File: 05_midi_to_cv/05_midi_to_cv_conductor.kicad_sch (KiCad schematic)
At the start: 21 parts, among them J1 MIDI IN 1, J2 MIDI IN 2, J3 MIDI IN 3, J5 Midi Fast Bus, U1 NCP1117-5.0_SOT223, U2 SN74HCT125

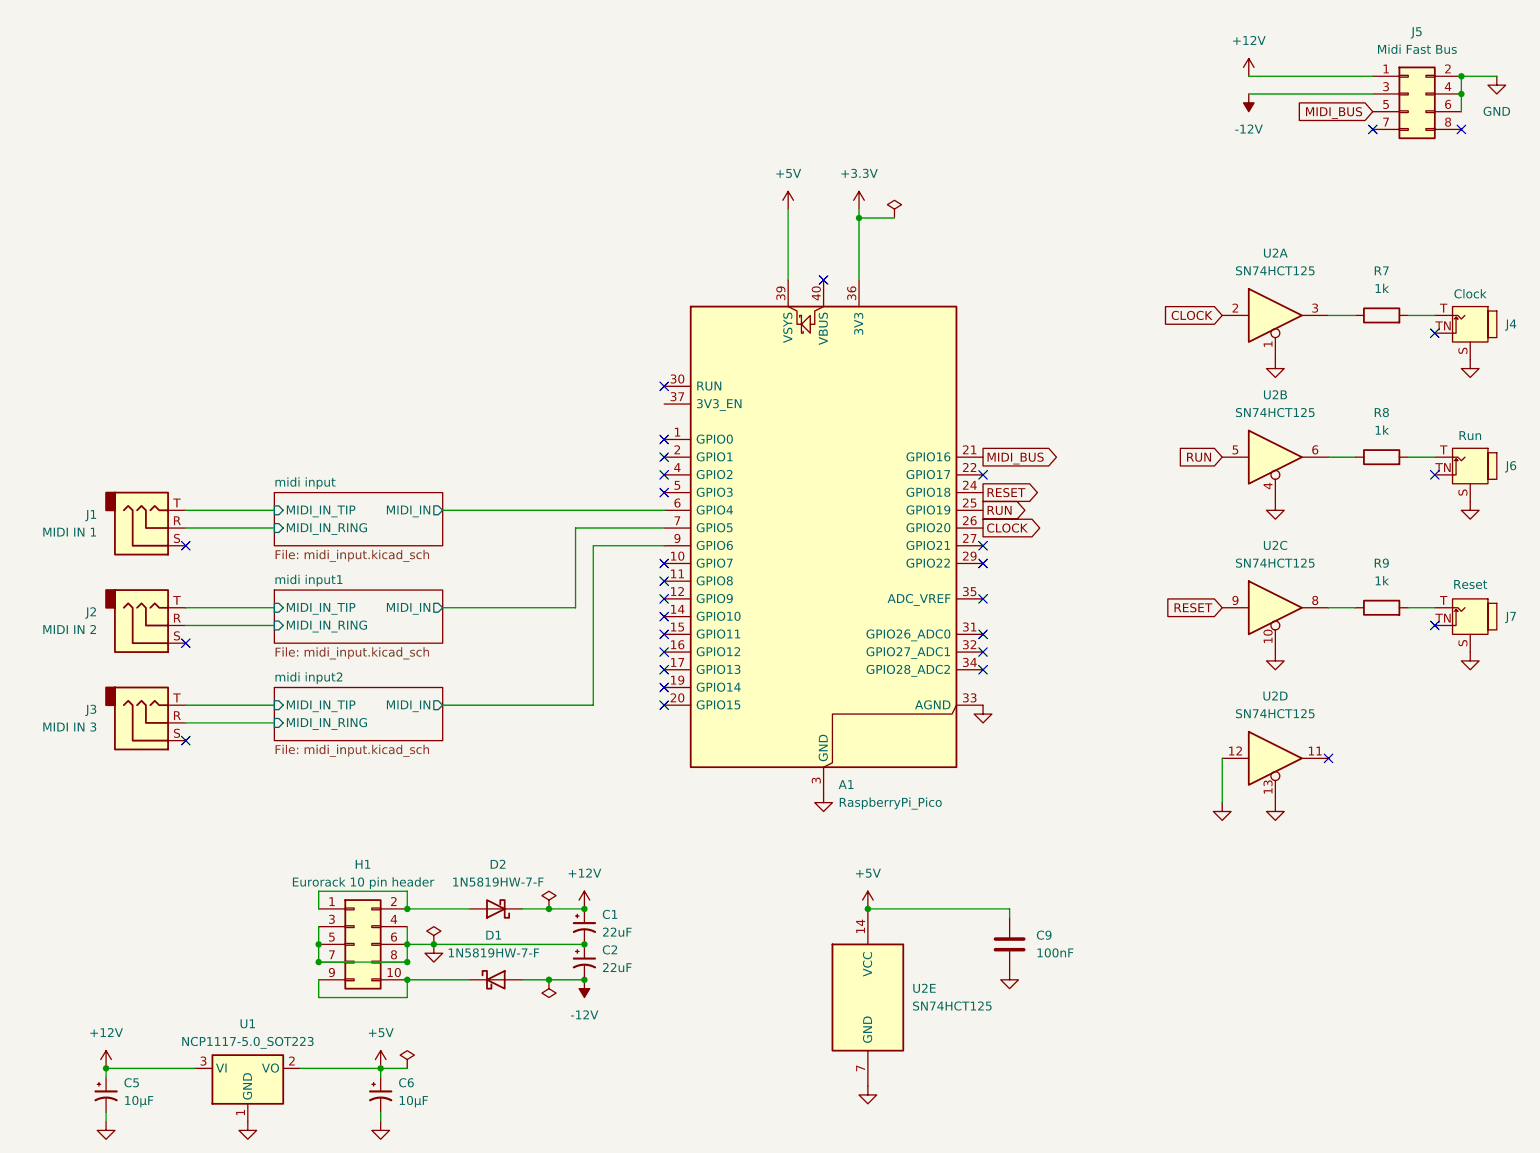
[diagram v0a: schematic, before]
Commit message: dual board 05
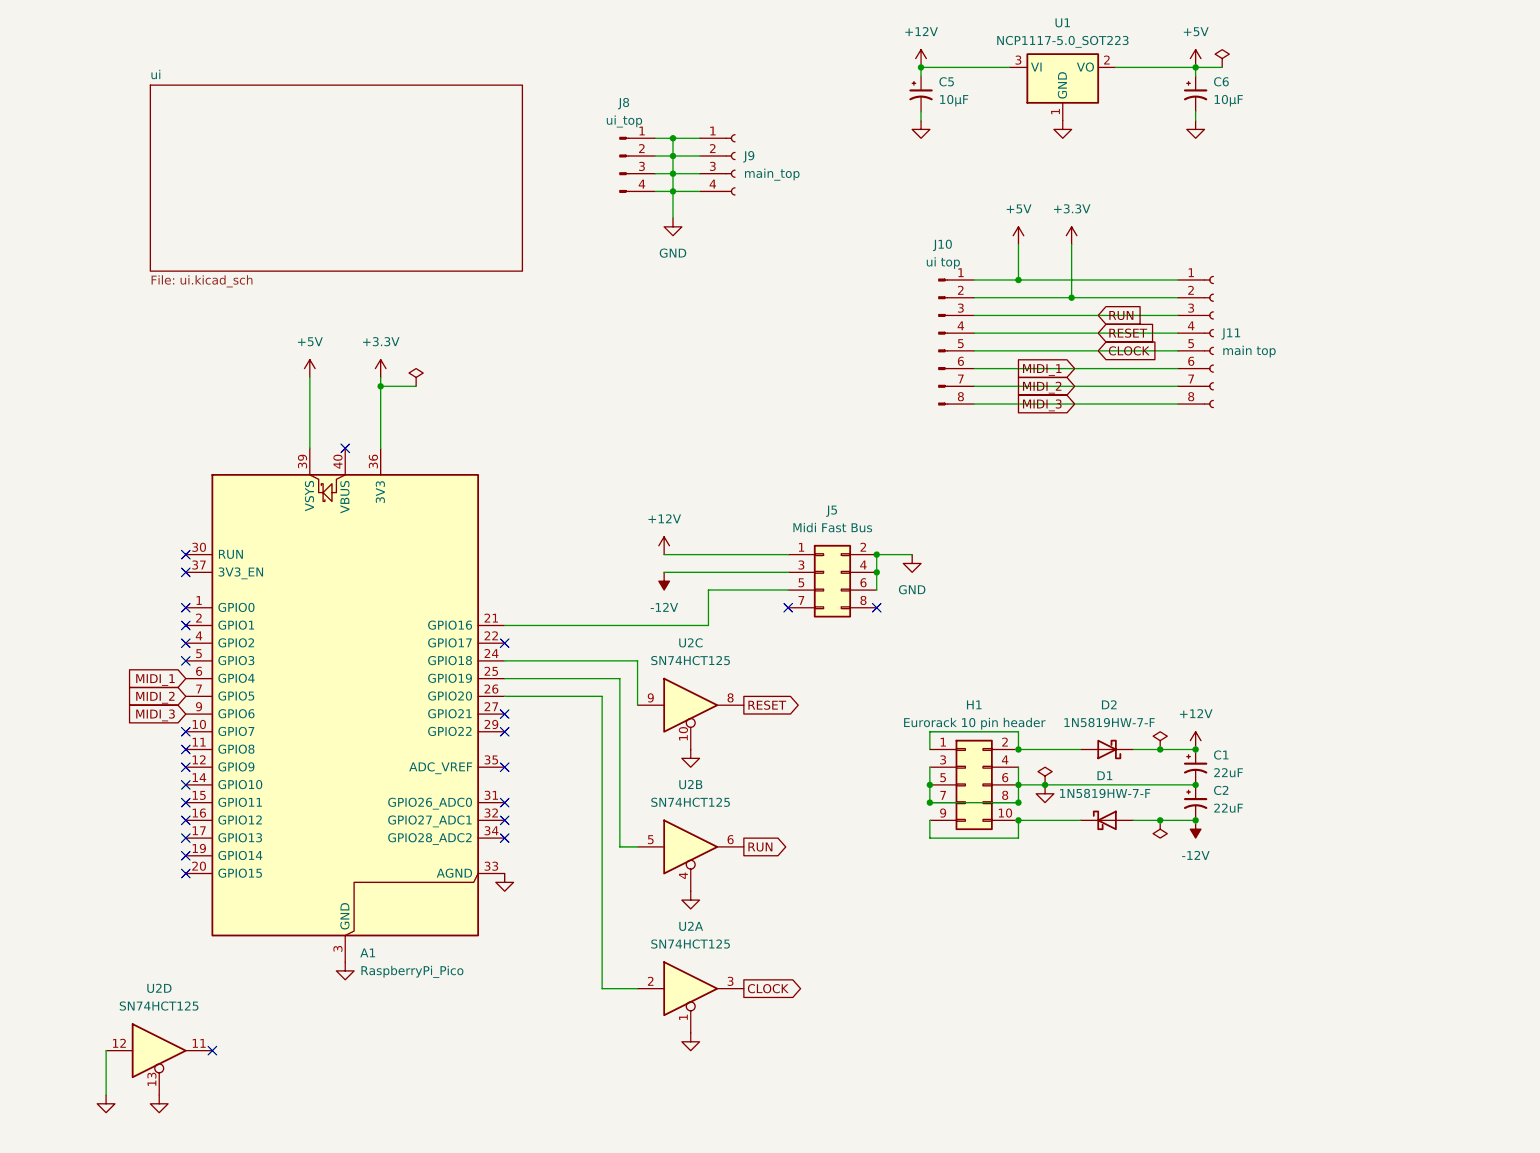
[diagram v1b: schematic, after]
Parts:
- removed C9: 100nF, cynthia:C SMD 0805, symbol Device:C
- removed J1: MIDI IN 1, cynthia:3.5mm jack stereo, symbol Connector_Audio:AudioJack3
- removed J2: MIDI IN 2, cynthia:3.5mm jack stereo, symbol Connector_Audio:AudioJack3
- removed J3: MIDI IN 3, cynthia:3.5mm jack stereo, symbol Connector_Audio:AudioJack3
- removed J4, J6, J7: (no value), cynthia:3.5mm thonk jack socket mono switched, symbol cynthia:3.5mm thonk jack socket mono switched
- removed R7, R8, R9: 1k, cynthia:R SMD 0805, symbol Device:R
- removed unit 5 of U2
- added J10: ui top, Connector_PinHeader_2.54mm:PinHeader_1x08_P2.54mm_Vertical, symbol Connector:Conn_01x08_Pin
- added J11: main top, Connector_PinSocket_2.54mm:PinSocket_1x08_P2.54mm_Vertical, symbol Connector:Conn_01x08_Socket
- added J8: ui_top, Connector_PinHeader_2.54mm:PinHeader_1x04_P2.54mm_Vertical, symbol Connector:Conn_01x04_Pin
- added J9: main_top, Connector_PinSocket_2.54mm:PinSocket_1x04_P2.54mm_Vertical, symbol Connector:Conn_01x04_Socket
- A1: footprint Module:RaspberryPi_Pico_Common_Unspecified -> Module:RaspberryPi_Pico_SMD_HandSolder
- J5: footprint 4ms_Connector:Pins_2x04_2.54mm_TH -> cynthia:Shrouded Header 8 pins
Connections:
- net +3.3V: now also J10.2 (Pin_2), J11.2 (Pin_2)
- net +5V: now also J10.1 (Pin_1), J11.1 (Pin_1)
- net CLOCK: now also U2.3, J10.5 (Pin_5), J11.5 (Pin_5); no longer A1.26 (GPIO20), U2.2
- net GND: now also J8.1 (Pin_1), J8.2 (Pin_2), J8.3 (Pin_3), J8.4 (Pin_4), J9.1 (Pin_1), J9.2 (Pin_2), J9.3 (Pin_3), J9.4 (Pin_4)
- net RESET: now also U2.8, J10.4 (Pin_4), J11.4 (Pin_4); no longer A1.24 (GPIO18), U2.9
- net RUN: now also U2.6, J10.3 (Pin_3), J11.3 (Pin_3); no longer A1.25 (GPIO19), U2.5
- net MIDI_BUS: no longer names the net of A1.21 (GPIO16), J5.5 (Pin_5)
- net midi input/MIDI_IN renamed MIDI_1
- net MIDI_1: now also J10.6 (Pin_6), J11.6 (Pin_6)
- net midi input1/MIDI_IN renamed MIDI_2
- net MIDI_2: now also J10.7 (Pin_7), J11.7 (Pin_7)
- net midi input2/MIDI_IN renamed MIDI_3
- net MIDI_3: now also J10.8 (Pin_8), J11.8 (Pin_8)
- new net: A1.26 (GPIO20), U2.2
- new net: A1.24 (GPIO18), U2.9
- new net: A1.25 (GPIO19), U2.5
- no-connect marks 31 -> 26
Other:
- removed sheet midi input
- removed sheet midi input1
- removed sheet midi input2
- added sheet ui (ui.kicad_sch)
- moved on the sheet: C1, C2, C5, C6, D1, D2, H1, U1
